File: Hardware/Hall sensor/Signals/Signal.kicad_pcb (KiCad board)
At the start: 2 copper layers, 72.6 x 35.6 mm, 46 parts, among them Q1 Q_NPN_Darlington_BEC, U1 Signals_MCC, U2 LM324, U3 LM324, U4 LM324

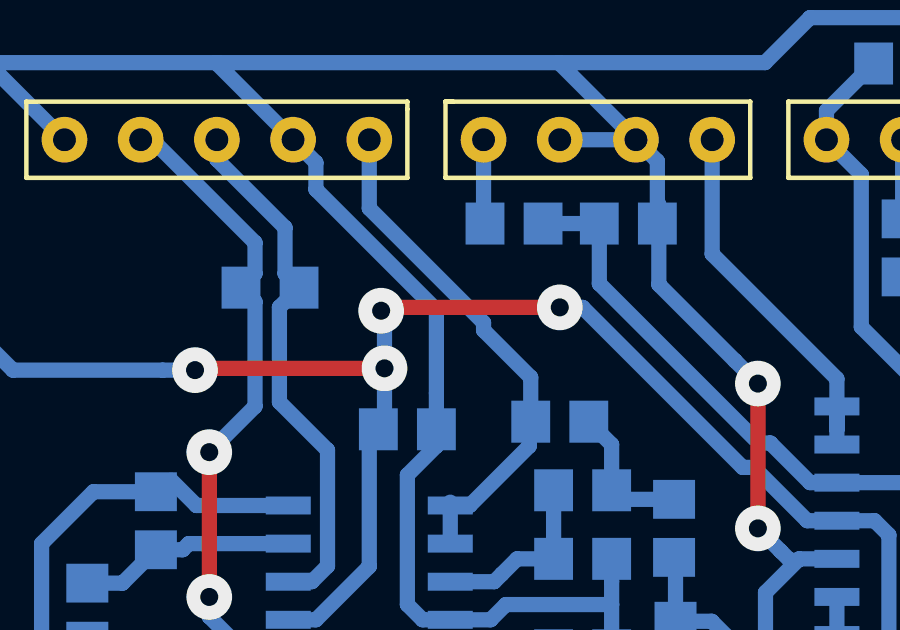
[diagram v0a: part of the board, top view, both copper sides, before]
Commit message: Updated fabrication outputs _Updated shunt signals PDF schematic,PDF PCB, GERBER PCB,Drill PCB_ _Updated shunt cuk PDF schematic,PDF PCB, GERBER PCB,Drill PCB_ _Updated hall signals PDF schematic,PDF PCB, GERBER PCB,Drill PCB_ _Updated hall cuk PDF schematic,PDF PCB, GERBER PCB,Drill PCB_
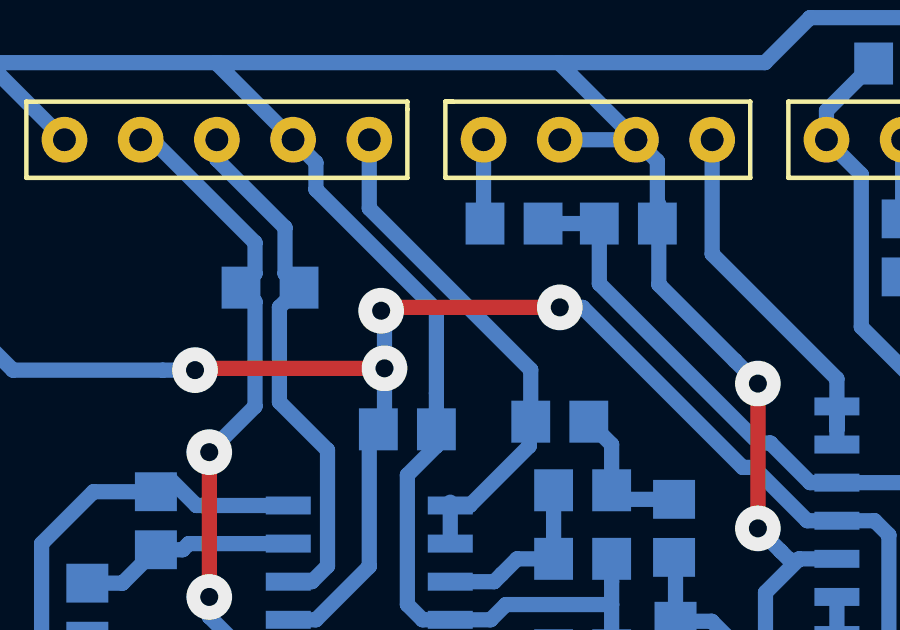
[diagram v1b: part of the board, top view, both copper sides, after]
